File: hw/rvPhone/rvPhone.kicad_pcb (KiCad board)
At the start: 4 copper layers, 135 x 70 mm, 251 parts, among them J1 USB_OTG, J2 BATT, J201 Modem, J202 SIM_Card, J203 Motor, J204 Camera, J205 Micro_SD_Card, J3 SJ-3571N, J301 iMX8, J302 Prog, J401 Touch, J402 Display, SW1 RESET, SW2 WAKE, SW201 BOOT, U1 BQ25895, U10 74HC595, U11 ICS-43434, U12 MAX98357A, U13 MAX98357A, U14 SN74LVC1G04DRY, U15 SN74LVC1G3157DRY, U2 TPS62293, U201 ESP32-WROOM, U202 SN74CBTLV3125RGY, U203 TXB0104RGY, U204 TXB0104RGY, U205 DRV2605L, U206 TPS22917, U207 SN74LVC2G66DCU, U208 SN74CBTLV3126RGY, U209 LSM9DS1, U3 TPS630250, U4 E310-G002, U401 FAN5333BSX, U402 SN74LVC3G06DCU, U403 BT815Q, U404 IS25LP128-JKLE, U405 DS90C185, U406 TS3DV520E, U407 TXS0104ERGY, U408 TXS0104ERGY, U409 SN74LVC2G06DRY, U5 IS25LP128-JKLE, U6 TMUX1574RSV, U7 74HC00, U8 74HC00, U9 74HC595, X1 SiT1533, Y1 16MHz, Y401 12MHz

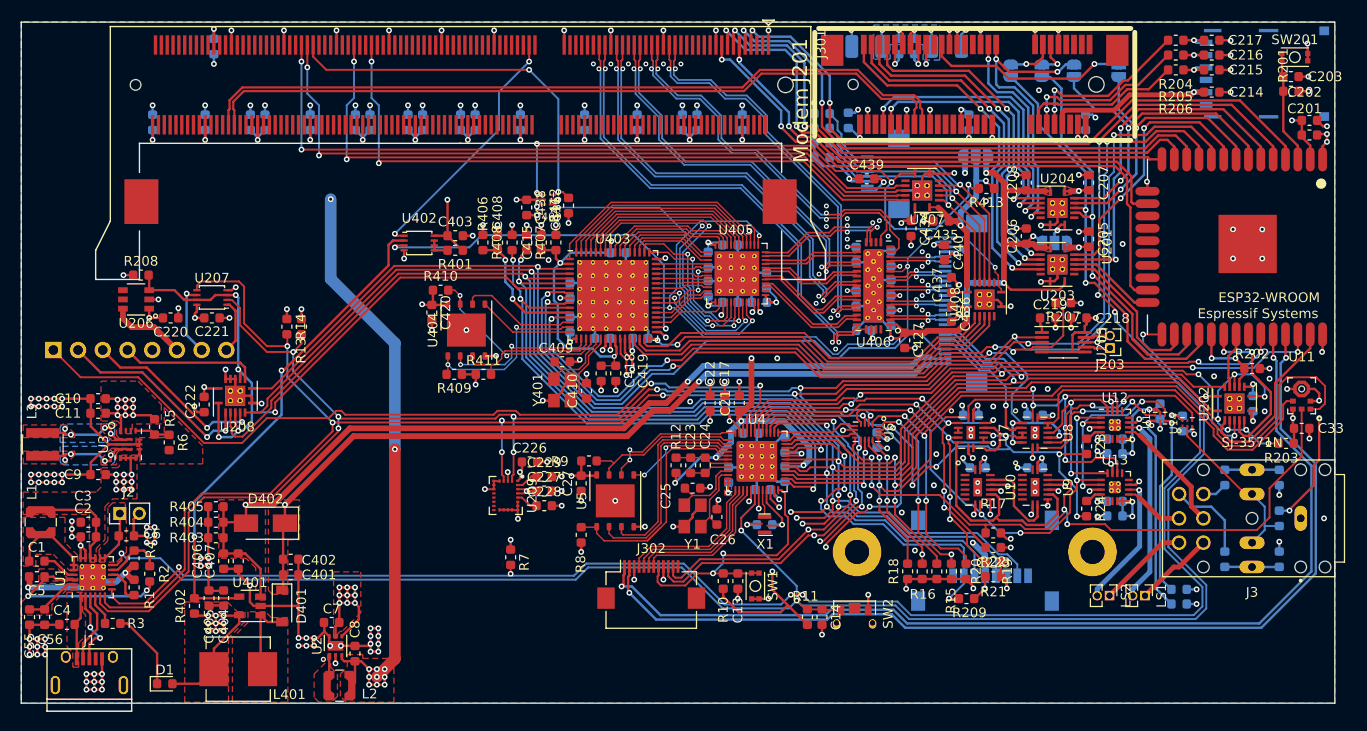
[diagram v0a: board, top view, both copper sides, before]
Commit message: rev2 board
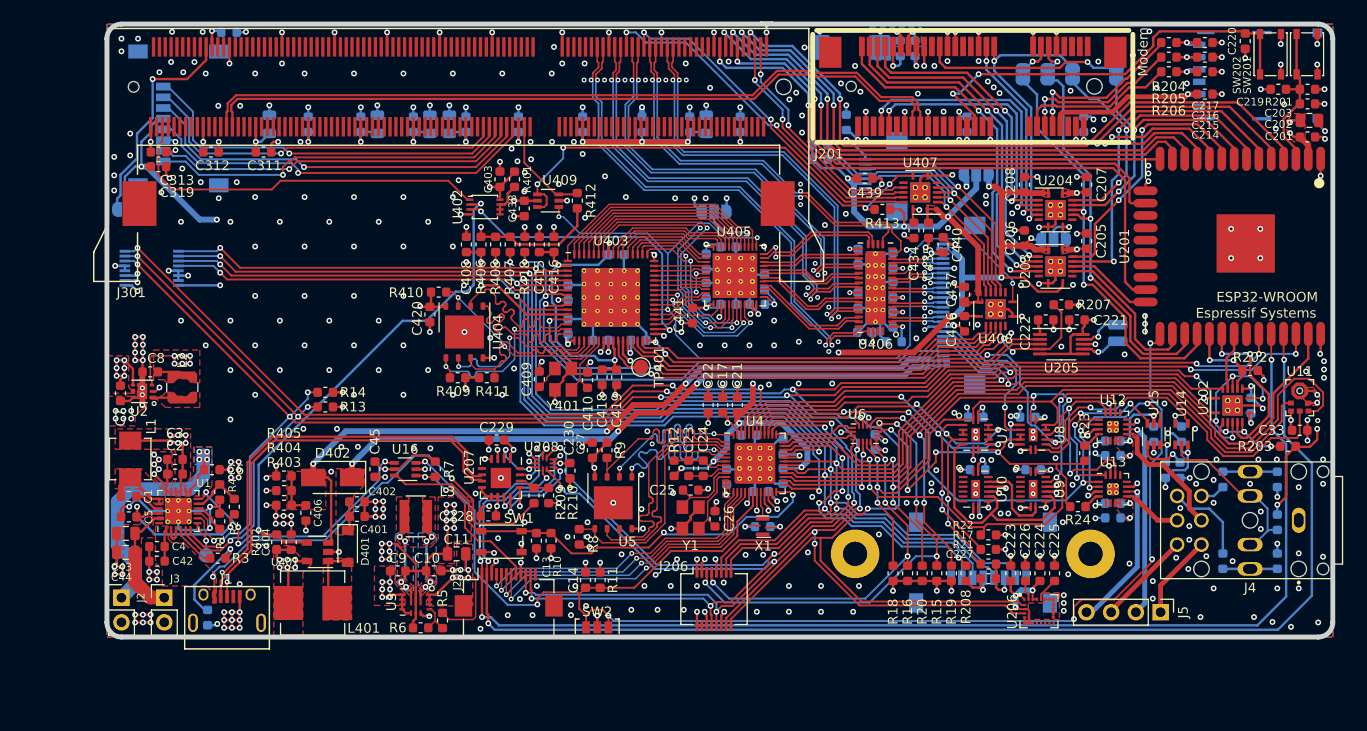
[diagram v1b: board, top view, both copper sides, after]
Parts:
- removed the C221 at (116.8, 102.2)
- removed the C222 at (116.0, 111.1)
- removed C405, C407: 27pF, Capacitor_SMD:C_0603_1608Metric
- removed C55, C56: 22uF, Capacitor_SMD:C_0603_1608Metric
- removed J302: Prog, Connector_FFC-FPC:Hirose_FH12-12S-0.5SH_1x12-1MP_P0.50mm_Horizontal
- removed LS1, LS2: Speaker, Connector_PinHeader_1.27mm:PinHeader_1x02_P1.27mm_Vertical
- removed the R208 at (109.5, 97.8)
- removed the R414 at (179.5, 82.7)
- removed R417: 100K, Resistor_SMD:R_0603_1608Metric
- removed U209: LSM9DS1, Package_LGA:LGA-24L_3x3.5mm_P0.43mm
- added C218: 470uF, Capacitor_Tantalum_SMD:CP_EIA-7343-31_Kemet-D, B.Cu at (182.4, 74.4)
- added C219: 10nF, Capacitor_SMD:C_0603_1608Metric, F.Cu at (226.4, 78.7)
- added C230: 0.1uF, Capacitor_SMD:C_0603_1608Metric, F.Cu at (153.6, 117.9)
- added C319: 0.1uF, Capacitor_SMD:C_0603_1608Metric, F.Cu at (111.3, 86.7)
- added C42: 10uF, Capacitor_SMD:C_0603_1608Metric, F.Cu at (111.2, 127.2)
- added C43: 22uF, Capacitor_SMD:C_0805_2012Metric, F.Cu at (108.0, 124.3)
- added C44: 22uF, Capacitor_SMD:C_0805_2012Metric, F.Cu at (108.0, 126.3)
- added C441: 10uF, Capacitor_SMD:C_0603_1608Metric, F.Cu at (166.2, 102.0)
- added C45: 0.1uF, Capacitor_SMD:C_0603_1608Metric, F.Cu at (133.6, 117.8)
- added J206: Expansion, Connector_Molex:Molex_SlimStack_54722-0164_2x08_P0.50mm_Vertical, F.Cu at (168.4, 131.1)
- added J207: Camera, Connector_Molex:Molex_SlimStack_54722-0164_2x08_P0.50mm_Vertical, B.Cu at (110.6, 97.1)
- added J305: Micro_SD_Card, footprints:microSD, B.Cu at (113.3, 81.7)
- added J4: SJ-3571N, footprints:SJ-3571N, F.Cu at (223.5, 123.0)
- added J5: SPEAKER, Connector_PinHeader_2.54mm:PinHeader_1x04_P2.54mm_Vertical, F.Cu at (214.3, 132.4)
- added JP301: ALT_BOOT, Jumper:SolderJumper-2_P1.3mm_Open_RoundedPad1.0x1.5mm, B.Cu at (107.7, 91.0)
- added JP402: VOD_SEL, Jumper:SolderJumper-3_P1.3mm_Open_RoundedPad1.0x1.5mm, B.Cu at (168.4, 91.3)
- added R209: 4.7K, Resistor_SMD:R_0603_1608Metric, F.Cu at (149.9, 120.5)
- added R210: 10K, Resistor_SMD:R_0603_1608Metric, F.Cu at (151.4, 120.5)
- added R418: 100K, Resistor_SMD:R_0603_1608Metric, F.Cu at (148.9, 94.7)
- added SW202: PERST, Button_Switch_SMD:SW_SPST_PTS810, F.Cu at (225.6, 75.1)
- added TP1: BQ_INT, TestPoint:TestPoint_Pad_D1.5mm, B.Cu at (116.2, 126.6)
- added TP401: AUDIO, TestPoint:TestPoint_Pad_D1.5mm, F.Cu at (160.9, 107.2)
- added U16: SN74LVC2G07DCK, Package_TO_SOT_SMD:Texas_R-PDSO-G6, F.Cu at (136.7, 117.8)
- C10: value 22uF -> 10uF
- C11: value 22uF -> 47uF; footprint Capacitor_SMD:C_0603_1608Metric -> Capacitor_SMD:C_0805_2012Metric
- C202: value 10uF -> 22uF; footprint Capacitor_SMD:C_0603_1608Metric -> Capacitor_SMD:C_0805_2012Metric
- C203: value 0.1uF -> 1uF
- C220: value 1uF -> 10nF
- C224: value 470uF -> 0.1uF; footprint Capacitor_Tantalum_SMD:CP_EIA-3528-21_Kemet-B -> Capacitor_SMD:C_0603_1608Metric; moved to F.Cu
- C225: value 470uF -> 0.01uF; footprint Capacitor_Tantalum_SMD:CP_EIA-3528-21_Kemet-B -> Capacitor_SMD:C_0603_1608Metric; moved to F.Cu
- C228: value 0.01uF -> 0.1uF
- C25, C26: value 12pF -> 10pF
- C311, C312, C313: moved to F.Cu
- C314, C315, C316, C317, C318: footprint Capacitor_SMD:C_0603_1608Metric -> Capacitor_SMD:C_0805_2012Metric
- C409, C410: value 18pF -> 10pF
- C427, D1: moved to B.Cu
- J2: footprint Connector_PinHeader_2.00mm:PinHeader_1x02_P2.00mm_Vertical -> Connector_PinHeader_2.54mm:PinHeader_1x02_P2.54mm_Vertical
- J203: footprint Connector_PinHeader_1.27mm:PinHeader_1x02_P1.27mm_Vertical -> footprints:SolderWirePad_1x02_SMD_1x2mm; moved to B.Cu
- J204: value Camera -> Micro_SD_Card; footprint Connector_PinHeader_2.54mm:PinHeader_1x08_P2.54mm_Vertical -> footprints:microSD
- J205: value Micro_SD_Card -> Prog; footprint footprints:microSD -> Connector_FFC-FPC:Hirose_FH12-12S-0.5SH_1x12-1MP_P0.50mm_Horizontal; moved to F.Cu
- J3: value SJ-3571N -> +5V; footprint footprints:SJ-3571N -> Connector_PinHeader_2.54mm:PinHeader_1x02_P2.54mm_Vertical
- L1: footprint footprints:L_Coilcraft_LPS3015 -> Inductor_SMD:L_Vishay_IHLP-1616
- R23: value 2K -> 2.2K
- R24: value 210K -> 255K
- R28, R29: value 100K -> 50K
- R405: value R -> 68R
- R414: renamed from R415; value 1K -> R
- R415: renamed from R416; value 1K -> R
- R7: value 10K -> 100K
- SW1, SW201: footprint footprints:Panasonic_EVPBB -> Button_Switch_SMD:SW_SPST_PTS810
- SW2: footprint footprints:Panasonic_EVPAK -> footprints:Panasonic_EVPAE
- U14: value SN74LVC1G04DRY -> SN74LVC1G04DCK; footprint footprints:USON-6_1.45x1mm_P0.5mm -> footprints:Texas_R-PDSO-G5
- U15: value SN74LVC1G3157DRY -> SN74LVC1G3157DCK; footprint footprints:USON-6_1.45x1mm_P0.5mm -> Package_TO_SOT_SMD:Texas_R-PDSO-G6
- U205: value DRV2605L -> DRV2605LDGS
- U206: value TPS22917 -> LSM9DS1; footprint footprints:TPS22917 -> Package_LGA:LGA-24L_3x3.5mm_P0.43mm
- U207: value SN74LVC2G66DCU -> FT230XQ; footprint Package_SO:VSSOP-8_2.4x2.1mm_P0.5mm -> Package_DFN_QFN:QFN-16-1EP_4x4mm_P0.65mm_EP2.1x2.1mm
- U208: value SN74CBTLV3126RGY -> TMUX154ERSW; footprint Package_DFN_QFN:Texas_S-PVQFN-N14_ThermalVias -> footprints:UQFN-10_1.4x1.8mm_P0.4mm
- U4: value E310-G002 -> FE310-G002
- U403: value BT815Q -> BT817Q; footprint Package_DFN_QFN:QFN-64-1EP_9x9mm_P0.5mm_EP7.3x7.3mm_ThermalVias -> Package_DFN_QFN:QFN-64-1EP_9x9mm_P0.5mm_EP6x6mm_ThermalVias
- U406: value TS3DV520E -> TS3DV520ERUA
- U409: value SN74LVC2G06DRY -> SN74LVC2G06DCK; footprint footprints:USON-6_1.45x1mm_P0.5mm -> Package_TO_SOT_SMD:Texas_R-PDSO-G6
- moved C220 114.1 mm to (223.0, 73.8), turned to 270 degrees
- moved J3 112.1 mm to (111.9, 130.9), turned to 0 degrees
- moved U206 98.2 mm to (201.8, 132.3), turned to 0 degrees
- moved J204 98.0 mm to (196.1, 127.3), turned to 180 degrees
- moved C225 57.5 mm to (203.4, 128.4), turned to 90 degrees
- moved C224 55.0 mm to (201.9, 128.4), turned to 90 degrees
- moved C226 52.2 mm to (200.4, 128.4), turned to 90 degrees
- moved J205 49.1 mm to (147.3, 130.4), turned to 0 degrees
- moved C227 46.5 mm to (196.6, 129.0)
- moved C11 39.6 mm to (141.9, 126.5)
- moved L3 39.1 mm to (137.8, 122.6), turned to 0 degrees
- moved C10 38.8 mm to (139.6, 128.2)
- moved C8 35.8 mm to (110.5, 107.8), turned to 180 degrees
- moved R5 35.7 mm to (140.5, 133.3)
- moved U207 35.0 mm to (146.5, 118.7), turned to 270 degrees
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- renumbered C218 to C221, C219 to C222, JP205 to JP204, JP204 to JP205, R209 to R208
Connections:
- net /disp/DISP_LVDS_CLK_N renamed /disp/DISP_LVDS_CLKN
- net /disp/DISP_LVDS_CLK_P renamed /disp/DISP_LVDS_CLKP
- net /disp/DS90_LVDS_A0_N renamed /disp/DS90_LVDS_A0N
- net /disp/DS90_LVDS_A0_P renamed /disp/DS90_LVDS_A0P
- net /disp/DS90_LVDS_A1_N renamed /disp/DS90_LVDS_A1N
- net /disp/DS90_LVDS_A1_P renamed /disp/DS90_LVDS_A1P
- net /disp/DS90_LVDS_A2_N renamed /disp/DS90_LVDS_A2N
- net /disp/DS90_LVDS_A2_P renamed /disp/DS90_LVDS_A2P
- net /disp/DS90_LVDS_A3_N renamed /disp/DS90_LVDS_A3N
- net /disp/DS90_LVDS_A3_P renamed /disp/DS90_LVDS_A3P
- net /disp/DS90_LVDS_CLK_N renamed /disp/DS90_LVDS_CLKN
- net /disp/DS90_LVDS_CLK_P renamed /disp/DS90_LVDS_CLKP
- net Net-(C203-Pad1) renamed /periph/ESP32.EN
- net RESET renamed /RESET
- net iMX8.LVDS0.A0_N renamed iMX8.LVDS0.A0N
- net iMX8.LVDS0.A0_P renamed iMX8.LVDS0.A0P
- net iMX8.LVDS0.A1_N renamed iMX8.LVDS0.A1N
- net iMX8.LVDS0.A1_P renamed iMX8.LVDS0.A1P
- net iMX8.LVDS0.A2_N renamed iMX8.LVDS0.A2N
- net iMX8.LVDS0.A2_P renamed iMX8.LVDS0.A2P
- net iMX8.LVDS0.A3_N renamed iMX8.LVDS0.A3N
- net iMX8.LVDS0.A3_P renamed iMX8.LVDS0.A3P
- net iMX8.LVDS0.CLK_N renamed iMX8.LVDS0.CLKN
- net iMX8.LVDS0.CLK_P renamed iMX8.LVDS0.CLKP
- C220 pad 1: +3V3 -> /periph/PERST
- C225 pad 1: +3V3 -> Net-(C225-Pad1)
- C226 pad 1: +3V3 -> Net-(C226-Pad1)
- C228 pad 1: Net-(C228-Pad1) -> +3V3
- C229 pad 1: Net-(C229-Pad1) -> +3V3
- C427 pad 1: +1V8 -> +3V3
- C428 pad 1: +1V8 -> +3V3
- C429 pad 1: +1V8 -> +3V3
- C430 pad 1: +1V8 -> +3V3
- C431 pad 1: +1V8 -> +3V3
- C432 pad 1: +1V8 -> +3V3
- C433 pad 1: +1V8 -> +3V3
- C439 pad 1: +3V3 -> +VCTP
- J1 pad 2: Net-(J1-Pad2) -> USB_D-
- J1 pad 3: Net-(J1-Pad3) -> USB_D+
- J1 pad 6: Net-(J1-Pad6) -> GND
- J201 pad 22: Net-(J201-Pad22) -> /periph/PERST
- J204 pad 1: GPIO_23 -> Net-(J204-Pad1)
- J204 pad 2: /periph/CAM.MOSI -> SPI1.SS3
- J204 pad 3: /periph/CAM.MISO -> SPI1.MOSI
- J204 pad 4: /periph/CAM.SCK -> +3V3
- J204 pad 5: GND -> SPI1.SCK
- J204 pad 6: /periph/CAM.PWR -> GND
- J204 pad 7: /periph/CAM.SDA -> SPI1.MISO
- J204 pad 8: /periph/CAM.SCL -> Net-(J204-Pad8)
- J205 pad 1: Net-(J205-Pad1) -> ESP32.UART0.RXD
- J205 pad 2: SPI1.SS3 -> ESP32.UART0.TXD
- J205 pad 3: SPI1.MOSI -> GND
- J205 pad 4: +3V3 -> JTAG_TCK
- J205 pad 5: SPI1.SCK -> JTAG_TDO
- J205 pad 6: GND -> JTAG_TMS
- J205 pad 7: SPI1.MISO -> JTAG_TDI
- J205 pad 8: Net-(J205-Pad8) -> JTAG_TRST_N
- J205 pad 9: Net-(J205-Pad9) -> GND
- J3 pad 1: GND -> /BQ_PMID
- J3 pad 2: Net-(C39-Pad1) -> GND
- J301 pad 129: iMX8.I2C1.SCL -> Net-(J301-Pad129)
- J301 pad 135: iMX8.I2C1.SDA -> Net-(J301-Pad135)
- J301 pad 149: iMX8.GPIO3.IO13 -> Net-(J301-Pad149)
- J301 pad 151: iMX8.GPIO3.IO12 -> Net-(J301-Pad151)
- J301 pad 153: iMX8.GPIO3.IO11 -> Net-(J301-Pad153)
- J301 pad 185: Net-(J301-Pad185) -> /exp/ALT_BOOT
- J301 pad 200: Net-(J301-Pad200) -> iMX8.PWM1
- J301 pad 3: Net-(J301-Pad3) -> iMX8.GPIO5.IO29
- J301 pad 43: Net-(J301-Pad43) -> iMX8.I2C3.SCL
- J301 pad 49: Net-(J301-Pad49) -> iMX8.I2C3.SDA
- J301 pad 5: Net-(J301-Pad5) -> iMX8.GPIO5.IO28
- J301 pad 61: Net-(J301-Pad61) -> GND
- J301 pad 67: Net-(J301-Pad67) -> GND
- J301 pad 75: iMX8.PWM1 -> Net-(J301-Pad75)
- J301 pad 76: Net-(J301-Pad76) -> iMX8.GPIO3.IO7
- J301 pad 80: Net-(J301-Pad80) -> /exp/SD2_CLK
- J301 pad 82: Net-(J301-Pad82) -> /exp/SD2_CMD
- J301 pad 84: Net-(J301-Pad84) -> /exp/SD2_DAT0
- J301 pad 86: Net-(J301-Pad86) -> /exp/SD2_DAT1
- J301 pad 88: Net-(J301-Pad88) -> /exp/SD2_DAT2
- J301 pad 90: Net-(J301-Pad90) -> /exp/SD2_DAT3
- J401 pad 3: +3V3 -> +VCTP
- J402 pad 19: SPI1.MISO -> DISP_CS
- J402 pad 20: SPI1.MOSI -> SPI1.SCK
- J402 pad 21: SPI1.SCK -> SPI1.MOSI
- J402 pad 22: DISP_CS -> SPI1.MISO
- R412 pad 2: iMX8.GPIO3.IO13 -> iMX8.GPIO3.IO7
- R414 pad 1: +3V3 -> +VCTP
- R415 pad 1: +3V3 -> +VCTP
- R7 pad 2: ESP32.IO39 -> JTAG_TRST_N
- U1 pad 12: WAKE -> /BQ_QON
- U1 pad 2: Net-(J1-Pad3) -> Net-(U1-Pad2)
- U1 pad 23: Net-(C55-Pad1) -> /BQ_PMID
- U1 pad 3: Net-(J1-Pad2) -> Net-(U1-Pad2)
- U1 pad 7: ESP32.IO39 -> /BQ_INT
- U1 pad 8: GND -> +VSYS
- U14 pad 5: Net-(U14-Pad5) -> +3V3
- U201 pad 10: TMUX.I2C0.SCL -> Net-(U201-Pad10)
- U201 pad 11: TMUX.I2C0.SDA -> Net-(U201-Pad11)
- U201 pad 34: ESP32.RXD0 -> ESP32.UART0.RXD
- U201 pad 35: ESP32.TXD0 -> ESP32.UART0.TXD
- U201 pad 5: ESP32.IO39 -> Net-(U201-Pad5)
- U206 pad 2: GND -> TMUX.I2C0.SCL
- U206 pad 3: BT81X.GPIO0 -> +3V3
- U206 pad 4: Net-(U206-Pad4) -> TMUX.I2C0.SDA
- U206 pad 5: Net-(U206-Pad5) -> +3V3
- U206 pad 6: /periph/CAM.PWR -> +3V3
- U207 pad 1: /periph/CAM.SCL -> +3V3
- U207 pad 2: TMUX.I2C0.SCL -> /periph/USB_RXD
- U207 pad 3: BT81X.GPIO0 -> GND
- U207 pad 5: TMUX.I2C0.SDA -> Net-(U207-Pad5)
- U207 pad 6: /periph/CAM.SDA -> USB_D+
- U207 pad 7: BT81X.GPIO0 -> USB_D-
- U208 pad 1: BT81X.GPIO0 -> UART0.RXD
- U208 pad 10: BT81X.GPIO0 -> /periph/USB_CBUS1
- U208 pad 2: /periph/CAM.MOSI -> ESP32.UART0.RXD
- U208 pad 3: SPI1.MOSI -> /periph/USB_TXD
- U208 pad 4: BT81X.GPIO0 -> GND
- U208 pad 5: /periph/CAM.MISO -> /periph/USB_RXD
- U208 pad 6: SPI1.MISO -> ESP32.UART0.TXD
- U208 pad 7: GND -> UART0.TXD
- U208 pad 8: SPI1.SCK -> /periph/USB_CBUS0
- U208 pad 9: /periph/CAM.SCK -> +3V3
- U4 pad 38: UART0.RX -> UART0.RXD
- U4 pad 39: UART0.TX -> UART0.TXD
- U406 pad 1: +1V8 -> +3V3
- U406 pad 13: +1V8 -> +3V3
- U406 pad 22: +1V8 -> +3V3
- U406 pad 31: +1V8 -> +3V3
- U406 pad 4: +1V8 -> +3V3
- U406 pad 40: +1V8 -> +3V3
- U406 pad 7: +1V8 -> +3V3
- U407 pad 10: iMX8.GPIO3.IO11 -> iMX8.GPIO5.IO29
- U407 pad 11: iMX8.GPIO3.IO12 -> iMX8.GPIO5.IO28
- U407 pad 12: iMX8.I2C1.SDA -> iMX8.I2C3.SDA
- U407 pad 13: iMX8.I2C1.SCL -> iMX8.I2C3.SCL
- U409 pad 3: iMX8.GPIO3.IO13 -> iMX8.GPIO3.IO7
- U7 pad 10: GPIO_18 -> Net-(U7-Pad10)
- U7 pad 11: /SPK_EN -> Net-(U7-Pad10)
- U7 pad 12: Net-(U7-Pad12) -> GPIO_18
- U7 pad 13: PWM1.2 -> GPIO_18
- U7 pad 8: Net-(U7-Pad12) -> /SPK_EN
- U7 pad 9: GPIO_18 -> PWM1.2
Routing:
- net ESP32.IO39: track 198.5 -> 0.00 mm, vias 7 -> 0
- net ESP32.UART0.TXD: track 0.00 -> 135.8 mm, vias 0 -> 4
- net ESP32.UART0.RXD: track 0.00 -> 135.2 mm, vias 0 -> 4
- net ESP32.TXD0: track 103.9 -> 0.00 mm, vias 2 -> 0
- net ESP32.RXD0: track 103.3 -> 0.00 mm, vias 2 -> 0
- net UART0.TXD: track 0.00 -> 88.3 mm, vias 0 -> 6
- net UART0.RXD: track 0.00 -> 87.9 mm, vias 0 -> 6
- net iMX8.GPIO3.IO11: track 74.6 -> 0.00 mm, vias 2 -> 0
- net iMX8.GPIO3.IO12: track 73.9 -> 0.00 mm, vias 2 -> 0
- net +1V8: track 201.3 -> 127.8 mm, vias 33 -> 23
- net iMX8.I2C1.SDA: track 71.2 -> 0.00 mm, vias 2 -> 0
- net iMX8.I2C1.SCL: track 68.3 -> 0.00 mm, vias 2 -> 0
- net +3V3: track 196.3 -> 247.0 mm, vias 73 -> 76
- net /periph/PERST: track 0.00 -> 43.3 mm, vias 0 -> 2
- net USB_D+: track 0.00 -> 43.2 mm, vias 0 -> 2
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- added copper zone on B.Cu, net +1V8
- added copper zone on F.Cu, net +VCTP
- added copper zone on F.Cu, net /BQ_PMID
- added copper zone on F.Cu, net /SPK_L_HP+
- added copper zone on F.Cu, net /SPK_R_HP_+
- added copper zone on B.Cu, net DISP_LED_A
- added copper zone on B.Cu, net DISP_LED_K
- added copper zone on PWR, net GND
- added copper zone on B.Cu, net Net-(C6-Pad1)
- removed copper zone on F.Cu, net Net-(C5-Pad1)
- removed copper zone on F.Cu, net Net-(C55-Pad1)
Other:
- board size 135 x 70 mm -> 126 x 63 mm
- net class MODEM_USB removed
- net class USB added: clearance 0.2, trace_width 0.2, via_dia 0.6, via_drill 0.3
- net class USB2DIFF added: clearance 0.1524, trace_width 0.2288, via_dia 0.508, via_drill 0.254
- rule pad_to_mask_clearance: 0.045 -> 0.05
